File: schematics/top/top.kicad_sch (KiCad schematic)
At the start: 10 parts, among them J1 CLT-108-02-F-D-BE-K-TR, J2 Conn_01x04_Socket, U1 AHT20-F

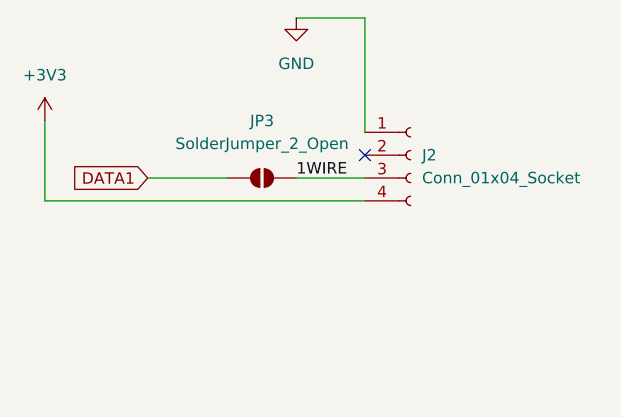
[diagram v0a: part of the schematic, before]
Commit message: Signed-off-by: Ray33ee <30669752+ray33ee@users.noreply.github.com>
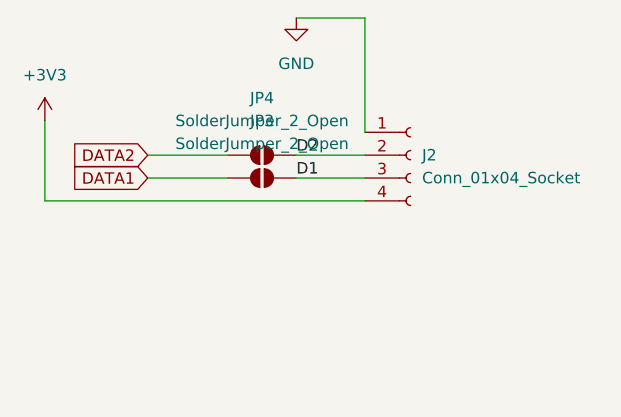
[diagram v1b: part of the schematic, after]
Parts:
- added JP4: SolderJumper_2_Open, Jumper:SolderJumper-2_P1.3mm_Open_RoundedPad1.0x1.5mm, symbol Jumper:SolderJumper_2_Open
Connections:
- net DATA2: now also JP4.1 (A)
- net D2: now reaches J2.2 (Pin_2)
- net D2: now also JP4.2 (B)
- net 1WIRE renamed D1
- no-connect marks 10 -> 9
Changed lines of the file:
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@@
-	)
-	(no_connect
-		(at 123.19 43.18)
 	)
 	(no_connect
@@
 	(wire
 		(pts
+			(xy 115.57 43.18) (xy 123.19 43.18)
+		)
+		(stroke
+			(width 0)
+			(type default)
+		)
+	)
+	(wire
+		(pts
 			(xy 222.25 59.69) (xy 210.82 59.69)
 		)
@@
 		(pts
 			(xy 205.74 101.6) (xy 215.9 101.6)
+		)
+		(stroke
+			(width 0)
+			(type default)
+		)
+	)
+	(wire
+		(pts
+			(xy 99.06 43.18) (xy 107.95 43.18)
 		)
 		(stroke
@@
 		)
 	)
-	(label "1WIRE"
+	(label "D1"
 		(at 115.57 45.72 0)
 		(effects
@@
 		)
 	)
+	(label "D2"
+		(at 115.57 43.18 0)
+		(effects
+			(font
+				(size 1.27 1.27)
+			)
+			(justify left bottom)
+		)
+	)
 	(global_label "BLUE"
 		(shape input)
@@
 		(property "Intersheetrefs" "${INTERSHEET_REFS}"
 			(at 181.2858 91.44 0)
+			(effects
+				(font
+					(size 1.27 1.27)
+				)
+				(justify right)
+				(hide yes)
+			)
+		)
+	)
+	(global_label "DATA2"
+		(shape input)
+		(at 99.06 43.18 180)
+		(fields_autoplaced yes)
+		(effects
+			(font
+				(size 1.27 1.27)
+			)
+			(justify right)
+		)
+		(property "Intersheetrefs" "${INTERSHEET_REFS}"
+			(at 90.4505 43.18 0)
 			(effects
 				(font
@@
 					(unit 1)
 				)
+			)
+		)
+	)
+	(symbol
+		(lib_id "Jumper:SolderJumper_2_Open")
+		(at 111.76 43.18 0)
+		(unit 1)
+		(exclude_from_sim no)
+		(in_bom yes)
+		(on_board yes)
+		(dnp no)
+		(fields_autoplaced yes)
+		(property "Reference" "JP4"
+			(at 111.76 36.83 0)
+			(effects
+				(font
+					(size 1.27 1.27)
+				)
+			)
+		)
+		(property "Value" "SolderJumper_2_Open"
+			(at 111.76 39.37 0)
+			(effects
+				(font
+					(size 1.27 1.27)
+				)
+			)
+		)
+		(property "Footprint" "Jumper:SolderJumper-2_P1.3mm_Open_RoundedPad1.0x1.5mm"
+			(at 111.76 43.18 0)
+			(effects
+				(font
+					(size 1.27 1.27)
+				)
+				(hide yes)
+			)
+		)
+		(property "Datasheet" "~"
+			(at 111.76 43.18 0)
+			(effects
+				(font
+					(size 1.27 1.27)
+				)
+				(hide yes)
+			)
+		)
+		(property "Description" "Solder Jumper, 2-pole, open"
+			(at 111.76 43.18 0)
+			(effects
+				(font
+					(size 1.27 1.27)
+				)
+				(hide yes)
+			)
+		)
+		(pin "1"
+		)
+		(pin "2"
+		)
+		(instances
+			(project "top"
+				(path "/32e629c0-9262-4821-96ad-ef677872d7ba"
+					(reference "JP4")
+					(unit 1)
+				)
